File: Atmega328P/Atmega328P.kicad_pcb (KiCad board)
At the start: 2 copper layers, 50.4 x 30.4 mm, 31 parts, among them J1 Conn_01x04_Pin, J2 Conn_01x09_Pin, J3 Conn_01x04_Pin, J4 Conn_02x03_Odd_Even, U1 24LC1025, U2 DS1337S_, U3 24LC1025, U4 ATMEGA328P-AU, Y1 32.768 KHz, Y2 16 MHz

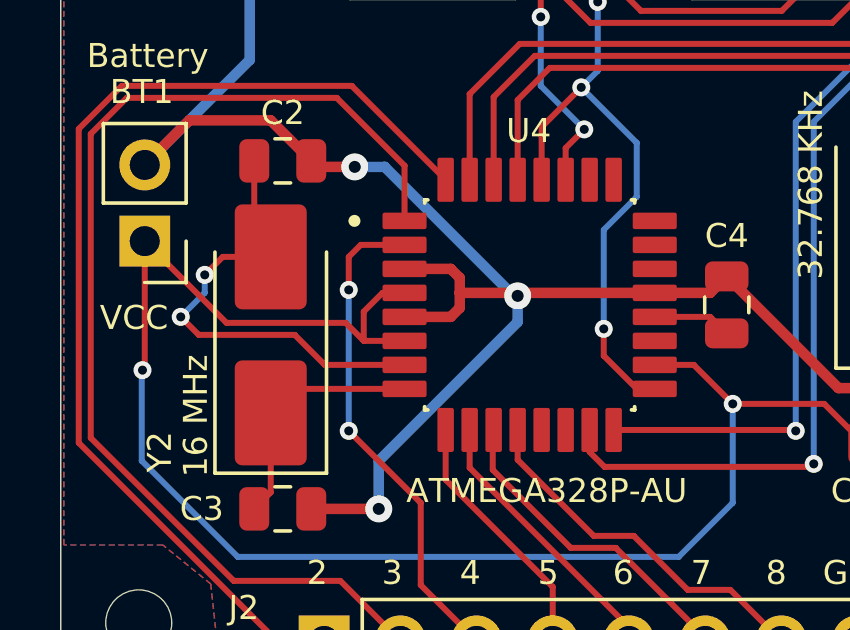
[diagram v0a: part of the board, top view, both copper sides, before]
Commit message: SCL Error- solver in schematic.
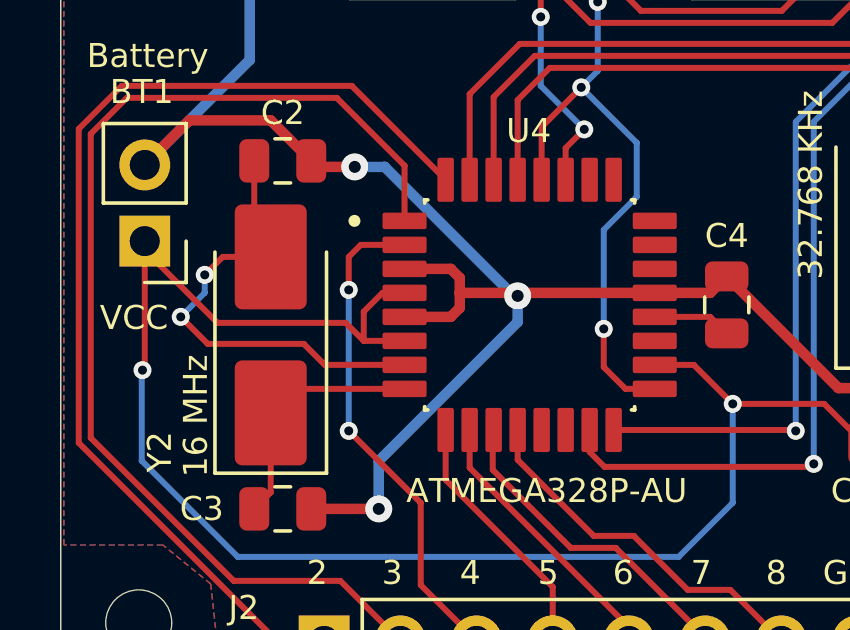
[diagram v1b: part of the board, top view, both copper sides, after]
